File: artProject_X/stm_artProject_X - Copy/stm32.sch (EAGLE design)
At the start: 20 parts

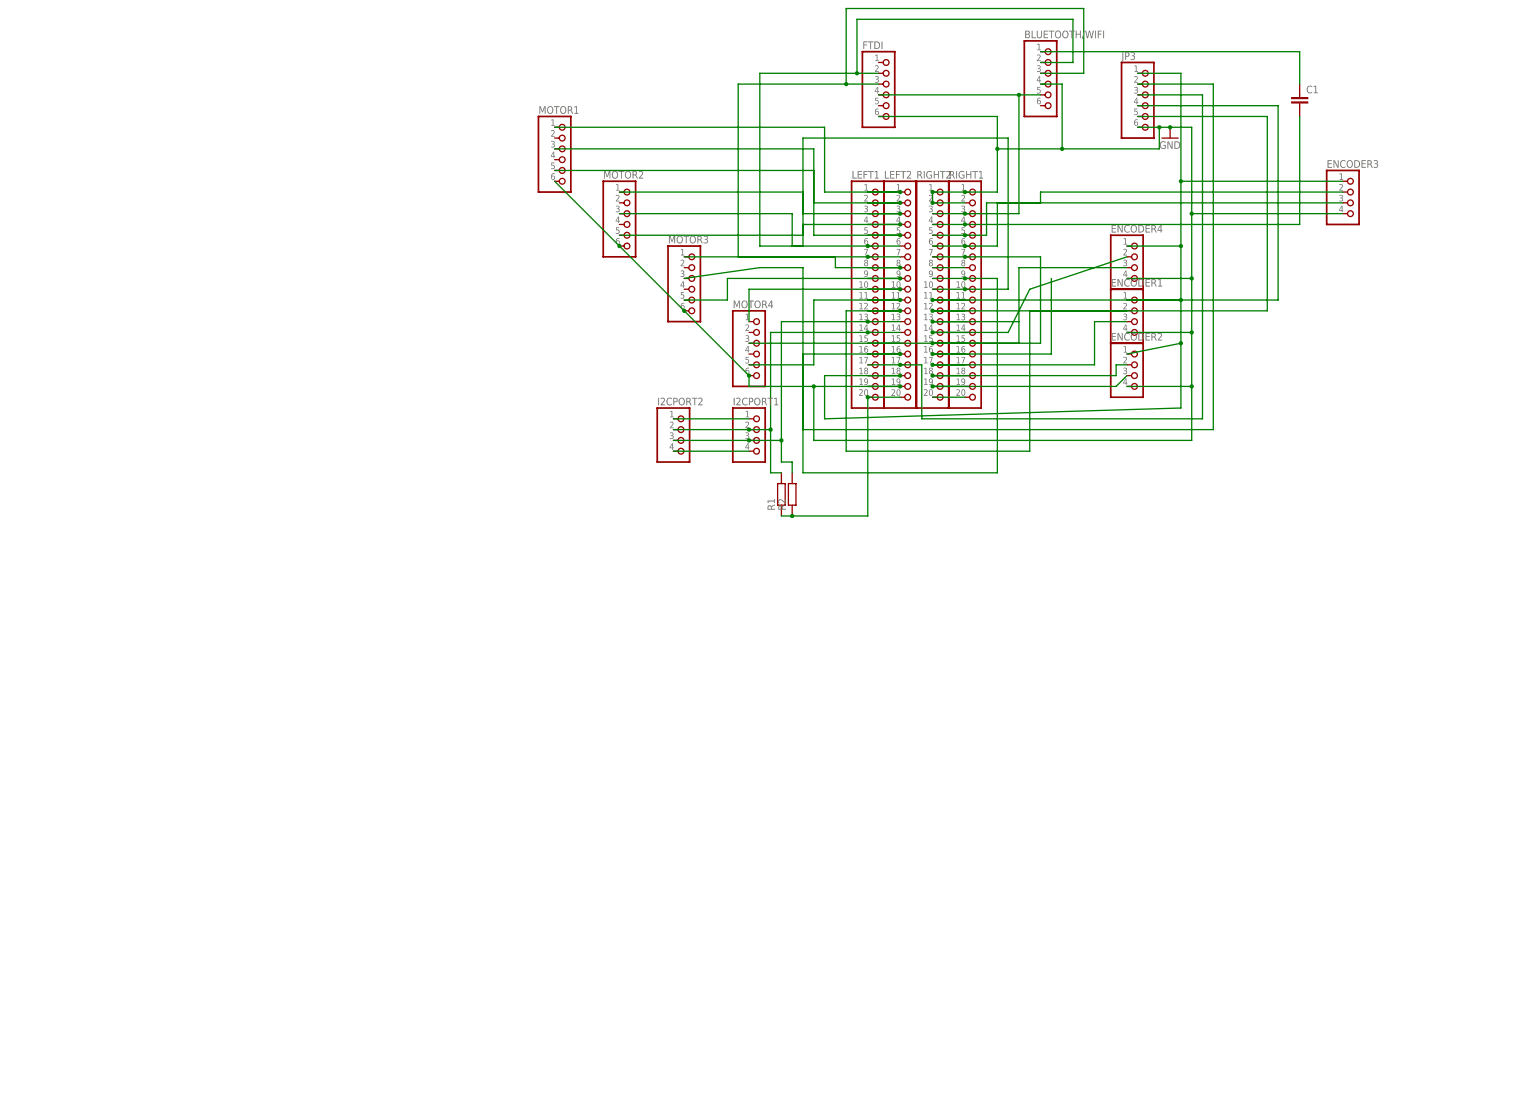
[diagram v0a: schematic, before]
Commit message: stm board complete files
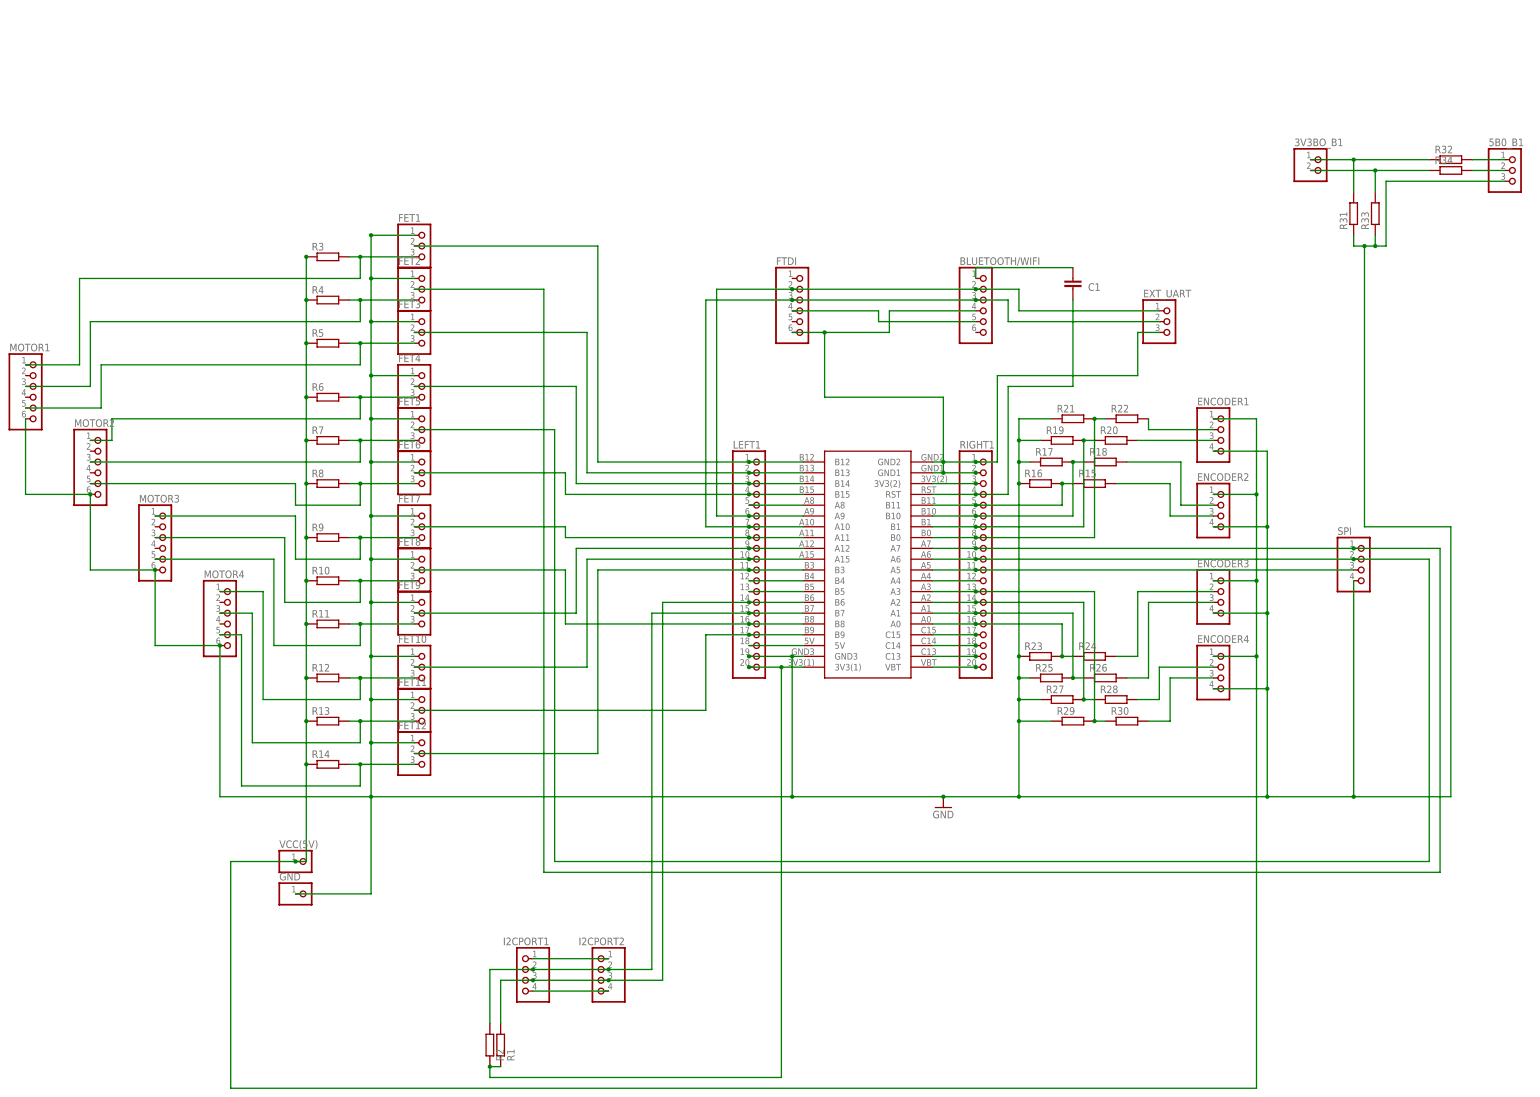
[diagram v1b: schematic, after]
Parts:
- removed JP3: (no value), pinhead:PINHD-1X6
- removed LEFT2, RIGHT2: (no value), pinhead:PINHD-1X20
- added 3V3BO_B1: (no value), pinhead:PINHD-1X2
- added 5B0_B1, EXT_UART, FET1, FET10, FET11, FET12, FET2, FET3, FET4, FET5, FET6, FET7, FET8, FET9: (no value), pinhead:PINHD-1X3
- added GND, VCC(5V): (no value), pinhead:PINHD-1X1
- added R10, R11, R12, R13, R14, R15, R16, R17, R18, R19, R20, R21, R22, R23, R24, R25, R26, R27, R28, R29, R3, R30, R31, R32, R33, R34, R4, R5, R6, R7, R8, R9: (no value), resistor:R-EU_0204/5
- added SPI: (no value), pinhead:PINHD-1X4
- added U$1: STM32THROUGH_HOLE, stm32:STM32THROUGH_HOLE
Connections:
- removed net ENCODER4: C1.2, RIGHT1.4, RIGHT2.4
- removed net N$38: ENCODER3.3, RIGHT1.6, RIGHT2.6
- new net 5V: ENCODER1.1, ENCODER2.1, ENCODER3.1, ENCODER4.1, R10.1, R11.1, R12.1, R13.1, R14.1, R3.1, R4.1, R5.1, R6.1, R7.1, R8.1, R9.1, VCC(5V).1
- new net B0: ENCODER1.2, R22.2
- new net B1: ENCODER1.3, R20.2
- new net N$29: R27.2, R28.1, RIGHT1.14, U$1.A2
- new net N$43: RIGHT1.3, U$1.3V3(2)
- new net N$44: C1.1, RIGHT1.4, U$1.RST
- new net N$45: R15.1, R16.2, RIGHT1.5, U$1.B11
- new net N$46: FET1.2, LEFT1.1, U$1.B12
- new net N$47: LEFT1.13, U$1.B5
- new net N$48: FET1.3, MOTOR1.1, R3.2
- new net N$49: FET2.3, MOTOR1.3, R4.2
- new net N$50: FET3.3, MOTOR1.5, R5.2
- new net N$51: FET4.3, MOTOR2.1, R6.2
- new net N$52: FET5.3, MOTOR2.3, R7.2
- new net N$53: FET6.3, MOTOR2.5, R8.2
- new net N$54: FET7.3, MOTOR3.1, R9.2
- new net N$55: FET8.3, MOTOR3.3, R10.2
- new net N$56: FET9.3, MOTOR3.5, R11.2
- new net N$57: FET11.3, MOTOR4.3, R13.2
- new net N$58: FET10.3, MOTOR4.1, R12.2
- new net N$59: FET12.3, MOTOR4.5, R14.2
- new net N$60: FET2.2, RIGHT1.9, SPI.1, U$1.A7
- new net N$63: R19.2, R20.1, RIGHT1.7, U$1.B1
- new net N$65: ENCODER3.2, R24.2
- new net N$66: ENCODER3.3, R26.2
- new net N$67: ENCODER4.2, R28.2
- new net N$68: ENCODER4.3, R30.2
- new net N$73: ENCODER2.2, R18.2
- new net N$74: ENCODER2.3, R15.2
- net GND: now also 5B0_B1.3, FET1.1, FET10.1, FET11.1, FET12.1, FET2.1, FET3.1, FET4.1, FET5.1, FET6.1, FET7.1, FET8.1, FET9.1, GND.1, R16.1, R17.1, R19.1, R21.1, R23.1, R25.1, R27.1, R29.1, R31.1, R33.1, SPI.4, U$1.GND3; no longer BLUETOOTH/WIFI.4, FTDI.6, JP3.6, LEFT2.19, RIGHT1.1, RIGHT1.2, RIGHT2.1, RIGHT2.2
- net N$1: now also 3V3BO_B1.1, R31.2, R32.1; no longer ENCODER1.1, ENCODER2.1, ENCODER3.1, ENCODER4.1, JP3.1, LEFT1.18, LEFT2.18
- net N$10: now also BLUETOOTH/WIFI.5, FTDI.4; no longer MOTOR3.3, RIGHT1.9, RIGHT2.9
- net N$11: now also FET10.2, LEFT1.10, U$1.A15; no longer LEFT1.8, LEFT2.8, MOTOR3.1
- net N$12: now also FET7.2, LEFT1.8, U$1.A11; no longer LEFT1.9, LEFT2.9, MOTOR3.5
- net N$13: now also FET9.2, LEFT1.9, U$1.A12; no longer LEFT1.10, LEFT2.10, MOTOR4.1
- net N$14: now also BLUETOOTH/WIFI.1, C1.2; no longer LEFT1.11, LEFT2.11, MOTOR4.5
- net N$15: now also FET12.2, LEFT1.11, U$1.B3; no longer ENCODER2.3, RIGHT1.19, RIGHT2.19
- net N$16: now also I2CPORT1.2, I2CPORT2.2, LEFT1.15, R2.2, U$1.B7; no longer ENCODER2.2, RIGHT1.18, RIGHT2.18
- net N$17: now also FET8.2, LEFT1.16, U$1.B8; no longer ENCODER1.3, RIGHT1.17, RIGHT2.17
- net N$18: now also FET11.2, LEFT1.17, U$1.B9; no longer ENCODER4.2, RIGHT1.14, RIGHT2.14
- net N$19: now also LEFT1.12, U$1.B4; no longer ENCODER4.3, RIGHT1.15, RIGHT2.15
- net N$2: now also FET3.2, LEFT1.2, U$1.B13; no longer BLUETOOTH/WIFI.1, C1.1
- net N$20: now also BLUETOOTH/WIFI.4, EXT_UART.3, FTDI.6, RIGHT1.1, RIGHT1.2, U$1.GND1, U$1.GND2; no longer RIGHT1.16, RIGHT2.16
- net N$21: now also 3V3BO_B1.2, R33.2, R34.1; no longer ENCODER1.2, LEFT1.12, LEFT2.12
- net N$22: now also RIGHT1.20, U$1.VBT; no longer RIGHT1.13, RIGHT2.13
- net N$23: now also RIGHT1.19, U$1.C13; no longer JP3.3, LEFT1.17, LEFT2.17
- net N$24: now also RIGHT1.18, U$1.C14; no longer JP3.2, LEFT1.16, LEFT2.16
- net N$25: now also RIGHT1.17, U$1.C15; no longer LEFT1.15, LEFT2.15
- net N$26: now also R23.2, R24.1, RIGHT1.16, U$1.A0; no longer MOTOR4.3, RIGHT1.7, RIGHT2.7
- net N$28: now also R25.2, R26.1, RIGHT1.15, U$1.A1; no longer BLUETOOTH/WIFI.2, FTDI.2, LEFT1.6, LEFT2.6
- net N$3: now also U$1.3V3(1); no longer LEFT2.20
- net N$30: now also I2CPORT1.3, I2CPORT2.3, U$1.B6; no longer I2CPORT1.2, I2CPORT2.2, LEFT2.14
- net N$31: now also R29.2, R30.1, RIGHT1.13, U$1.A3; no longer BLUETOOTH/WIFI.3, FTDI.3, LEFT1.7, LEFT2.7
- net N$32: now also RIGHT1.12, U$1.A4; no longer JP3.4, RIGHT1.11, RIGHT2.11
- net N$33: now also RIGHT1.11, SPI.3, U$1.A5; no longer JP3.5, RIGHT1.12, RIGHT2.12
- net N$34: now also 5B0_B1.1, R32.2; no longer I2CPORT1.3, I2CPORT2.3, LEFT1.13, LEFT2.13, R2.2
- net N$35: now also FET5.2, RIGHT1.10, SPI.2, U$1.A6; no longer BLUETOOTH/WIFI.5, FTDI.4, RIGHT1.3, RIGHT2.3
- net N$36: now also 5B0_B1.2, R34.2; no longer RIGHT1.8, RIGHT2.8
- net N$37: now also R21.2, R22.1, RIGHT1.8, U$1.B0; no longer ENCODER3.2, RIGHT1.5, RIGHT2.5
- net N$39: now also R17.2, R18.1, RIGHT1.6, U$1.B10; no longer RIGHT1.20, RIGHT2.20
- net N$4: now also FET4.2, LEFT1.3, U$1.B14; no longer LEFT1.1, LEFT2.1, MOTOR1.1
- net N$5: now also FET6.2, LEFT1.4, U$1.B15; no longer LEFT1.2, LEFT2.2, MOTOR1.5
- net N$6: now also LEFT1.5, U$1.A8; no longer LEFT1.3, LEFT2.3, MOTOR2.1
- net N$7: now also BLUETOOTH/WIFI.2, EXT_UART.1, FTDI.2, LEFT1.6, U$1.A9; no longer LEFT1.4, LEFT2.4, MOTOR2.5
- net N$8: now also LEFT1.18, U$1.5V; no longer LEFT1.5, LEFT2.5, MOTOR1.3
- net N$9: now also BLUETOOTH/WIFI.3, EXT_UART.2, FTDI.3, LEFT1.7, U$1.A10; no longer MOTOR2.3, RIGHT1.10, RIGHT2.10
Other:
- moved on the sheet: BLUETOOTH/WIFI, C1, ENCODER1, ENCODER2, ENCODER3, ENCODER4, FTDI, I2CPORT1, I2CPORT2, LEFT1, MOTOR1, MOTOR2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
